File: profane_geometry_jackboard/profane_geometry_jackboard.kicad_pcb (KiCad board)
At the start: 2 copper layers, 71.1 x 114.3 mm, 23 parts, among them J1 TriAmt, J11 NotchOut, J12 PulseAmt, J13 V/OCT, J14 PulseCV, J15 MixOut, J2 TriOut, J3 Conn_02x08_Counter_Clockwise, J4 Conn_01x12, J5 SquareAmt, J6 SquareOut, J7 Conn_01x12, J8 PulseOut, J9 PulseAmt

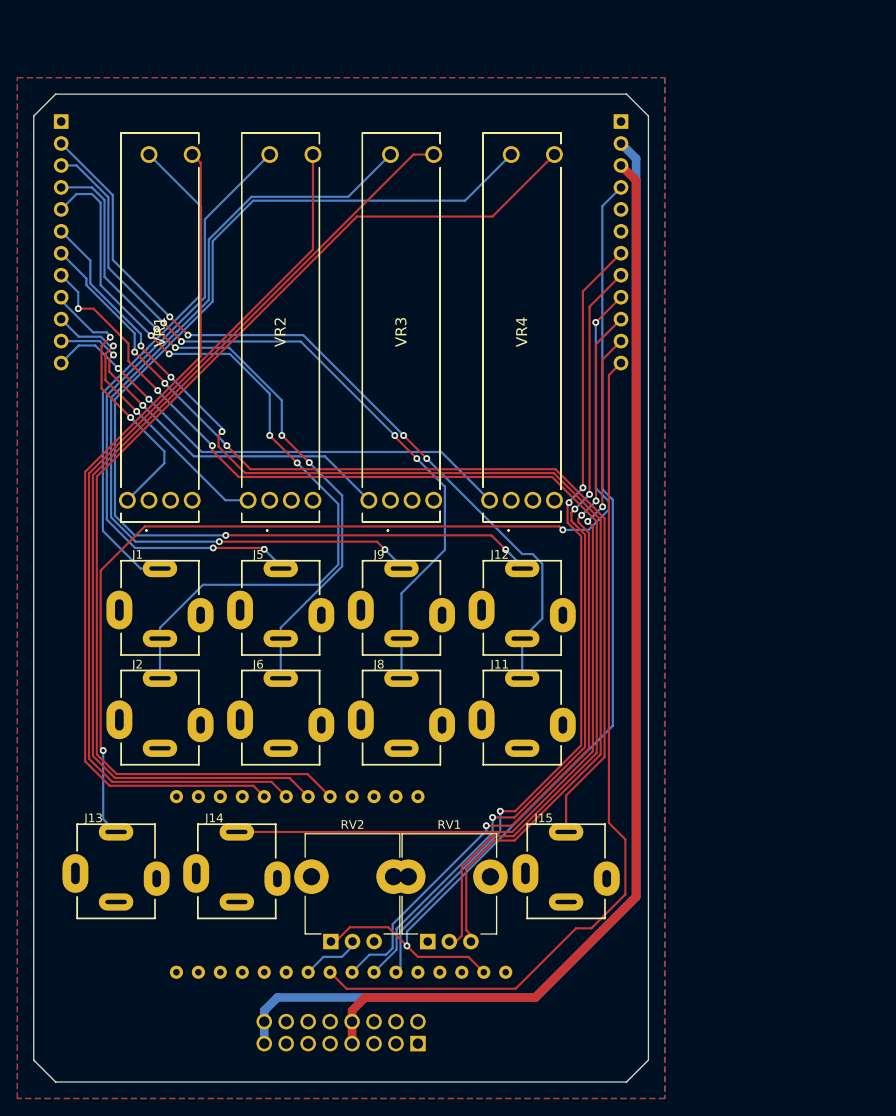
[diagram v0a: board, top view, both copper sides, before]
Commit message: update .gitignore, current kicad project
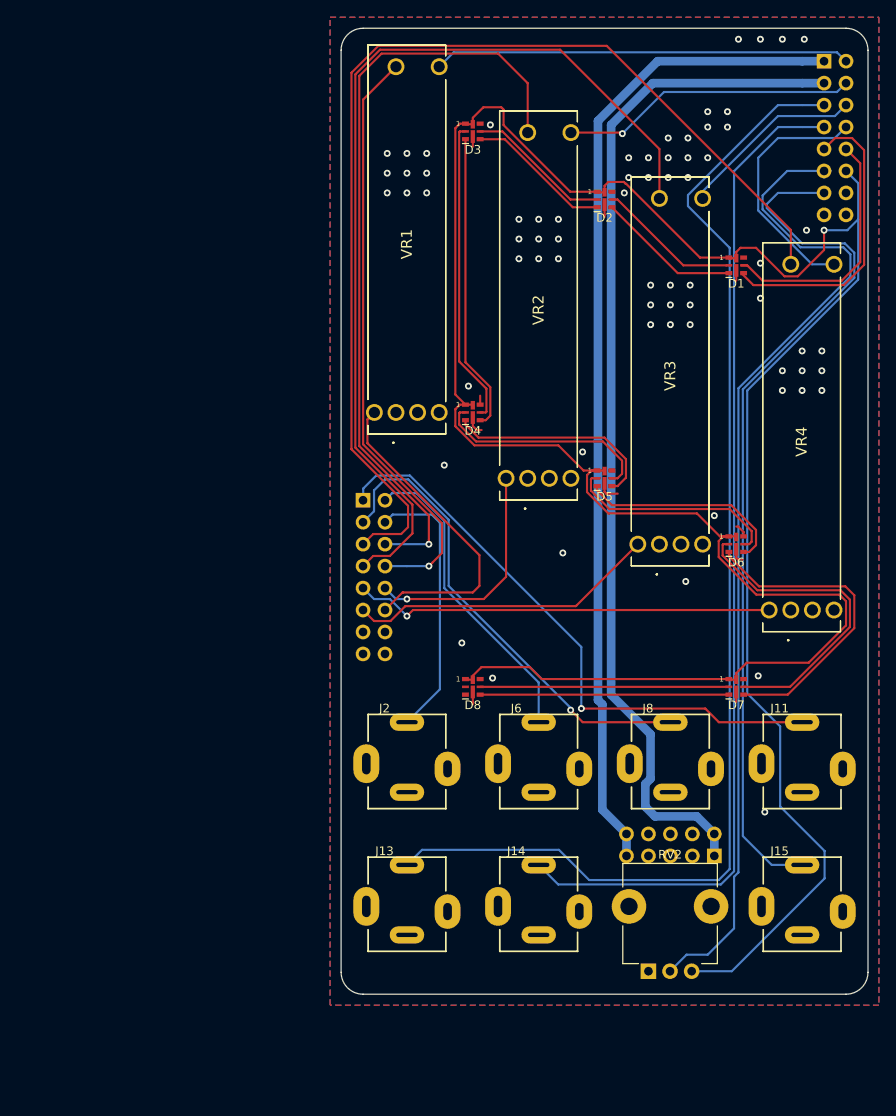
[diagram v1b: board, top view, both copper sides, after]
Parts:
- removed A1: Adafruit_Feather_M0_Express, profane_geometry_jackboard:Adafruit_Feather_M0_Express
- removed J12, J9: PulseAmt, profane_geometry_jackboard:Jack_3.5mm_QingPu_WQP-PJ301BM_Vertical
- removed J5: SquareAmt, profane_geometry_jackboard:Jack_3.5mm_QingPu_WQP-PJ301BM_Vertical
- removed J7: Conn_01x12, Connector_PinHeader_2.54mm:PinHeader_1x12_P2.54mm_Vertical
- removed REF**: OSHW-Logo2_7.3x6mm_SilkScreen, profane_geometry_jackboard:OSHW-Logo2_7.3x6mm_SilkScreen
- removed RV1: MixAtt, Potentiometer_THT:Potentiometer_TT_P0915N
- removed Ref**: Val**, profane_geometry_jackboard:zzzzzzzz_new
- added D1: APA102-2020, LED_SMD:LED-APA102-2020, F.Cu at (182.9, 73.2)
- added D2: APA102-2020, LED_SMD:LED-APA102-2020, F.Cu at (167.6, 65.5)
- added D3: APA102-2020, LED_SMD:LED-APA102-2020, F.Cu at (152.4, 57.7)
- added D4: APA102-2020, LED_SMD:LED-APA102-2020, F.Cu at (152.4, 90.2)
- added D5: APA102-2020, LED_SMD:LED-APA102-2020, F.Cu at (167.6, 97.8)
- added D6: APA102-2020, LED_SMD:LED-APA102-2020, F.Cu at (182.9, 105.4)
- added D7: APA102-2020, LED_SMD:LED-APA102-2020, F.Cu at (182.9, 121.9)
- added D8: APA102-2020, LED_SMD:LED-APA102-2020, F.Cu at (152.4, 121.9)
- J1: value TriAmt -> Conn_02x08_Odd_Even; footprint profane_geometry_jackboard:Jack_3.5mm_QingPu_WQP-PJ301BM_Vertical -> Connector_PinSocket_2.54mm:PinSocket_2x08_P2.54mm_Vertical; moved to B.Cu
- J3: value Conn_02x08_Counter_Clockwise -> Conn_02x08_Odd_Even; footprint profane_geometry_jackboard:Molex_02x08_2.54mm_Shrouded_Keyed -> Connector_PinSocket_2.54mm:PinSocket_2x08_P2.54mm_Vertical
- J4: value Conn_01x12 -> Conn_02x05_Odd_Even; footprint Connector_PinHeader_2.54mm:PinHeader_1x12_P2.54mm_Vertical -> Connector_PinHeader_2.54mm:PinHeader_2x05_P2.54mm_Vertical
- moved J3 128.6 mm to (193.0, 49.5), turned to 180 degrees
- moved J4 113.7 mm to (180.3, 141.5), turned to 90 degrees
- moved RV2 36.9 mm to (172.7, 154.8)
- moved J14 35.1 mm to (160.0, 147.3)
- moved VR4 34.7 mm to (189.2, 113.0)
- moved J13 33.9 mm to (144.8, 147.3)
- moved J11 32.8 mm to (190.5, 130.8)
- moved VR3 31.5 mm to (174.0, 105.4)
- moved J8 31.5 mm to (175.3, 130.8)
- moved VR1 30.3 mm to (143.5, 90.2)
- moved J6 30.3 mm to (160.0, 130.8)
- moved VR2 30.0 mm to (158.8, 97.8)
- moved J2 29.0 mm to (144.8, 130.8)
- moved J15 27.6 mm to (190.5, 147.3)
- moved J1 26.7 mm to (139.7, 100.3), turned to 180 degrees
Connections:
- J3 pad 1: Net-(J3-Pad1) -> /-12v-rack
- J3 pad 10: GND -> /rgb-scl
- J3 pad 11: GND -> /pulse-pot
- J3 pad 12: GND -> +3V3
- J3 pad 13: /+12v-rack -> /mix-out
- J3 pad 15: Net-(J3-Pad15) -> GND
- J3 pad 16: Net-(J3-Pad16) -> GND
- J3 pad 2: Net-(J3-Pad2) -> /tri-slider-led
- J3 pad 3: Net-(J3-Pad3) -> /+12v-rack
- J3 pad 4: /+12v-rack -> /square-slider-led
- J3 pad 5: GND -> /v_oct-cv
- J3 pad 6: GND -> /pulse-slider-led
- J3 pad 7: GND -> /pulse-cv
- J3 pad 8: /-12v-rack -> /notch-slider-led
- J3 pad 9: /-12v-rack -> /rgb-sda
- J4 pad 1: GND -> /+12v-rack
- J4 pad 10: /square-att -> /-12v-rack
- J4 pad 2: /notch-out -> /+12v-rack
- J4 pad 3: /pulse-out -> GND
- J4 pad 4: /square-out -> GND
- J4 pad 5: /tri-out -> GND
- J4 pad 6: /mix-pre -> GND
- J4 pad 7: /mix-out -> GND
- J4 pad 8: /mix-att -> GND
- J4 pad 9: /tri-att -> /-12v-rack
- RV2 pad 1: +3V3 -> GND
- RV2 pad 3: GND -> +3V3
- VR1 pad 2: /tri-att -> /tri-mix
- VR1 pad 3: Net-(J1-PadT) -> /tri-pre-out
- VR1 pad B1: /tri-led -> /tri-slider-led
- VR2 pad 2: /square-att -> /square-mix
- VR2 pad 3: Net-(J5-PadT) -> /square-pre-out
- VR2 pad B1: /square-led -> /square-slider-led
- VR3 pad 2: /pulse-att -> /pulse-mix
- VR3 pad 3: Net-(J9-PadT) -> /pulse-pre-out
- VR3 pad B1: /pulse-led -> /pulse-slider-led
- VR4 pad 2: /notch-att -> /notch-mix
- VR4 pad 3: Net-(J12-PadT) -> /notch-pre-out
- VR4 pad B1: /notch-led -> /notch-slider-led
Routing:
- net +3V3: track 119.0 -> 325.8 mm
- net /mix-pre: track 137.6 -> 0.00 mm, vias 3 -> 0
- net /mix-att: track 133.2 -> 0.00 mm, vias 3 -> 0
- net /notch-led: track 129.5 -> 0.00 mm
- net /notch-pre-out: track 0.00 -> 126.2 mm
- net Net-(J12-PadT): track 125.0 -> 0.00 mm, vias 2 -> 0
- net /pulse-led: track 114.1 -> 0.00 mm
- net /pulse-pre-out: track 0.00 -> 110.0 mm
- net /pulse-pot: track 7.15 -> 116.3 mm
- net /square-led: track 105.3 -> 0.00 mm
- net /pulse-scaled: track 102.3 -> 0.00 mm
- net /tri-led: track 98.6 -> 0.00 mm
- net Net-(J9-PadT): track 98.2 -> 0.00 mm, vias 2 -> 0
- net /SERCOM4[0]: track 96.3 -> 0.00 mm, vias 3 -> 0
- net /SERCOM4[1]: track 95.3 -> 0.00 mm, vias 3 -> 0
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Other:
- board size 71.1 x 114.3 mm -> 61 x 111.8 mm
- board text removed: "Profane Geometry Jackboard Rev1"
